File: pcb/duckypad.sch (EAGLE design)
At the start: 159 parts, among them IC2 REG1117, SW1 SPST_TACT-EVQQ2, SW2 SPST_TACT-EVQQ2, SW21 EC12E_SW, SW22 EC12E_SW, SW3 324_SW324_SWITCH_FOOT_HOLE, SW4 324_SW324_SWITCH_FOOT_HOLE, U1 USBC_16P, U2 USBC_16P, U3 ESP32-S3FN8, U5 W25Q32FVSS, X3 SM12B-SSR-H-TB, Y1 16MHz_12pF

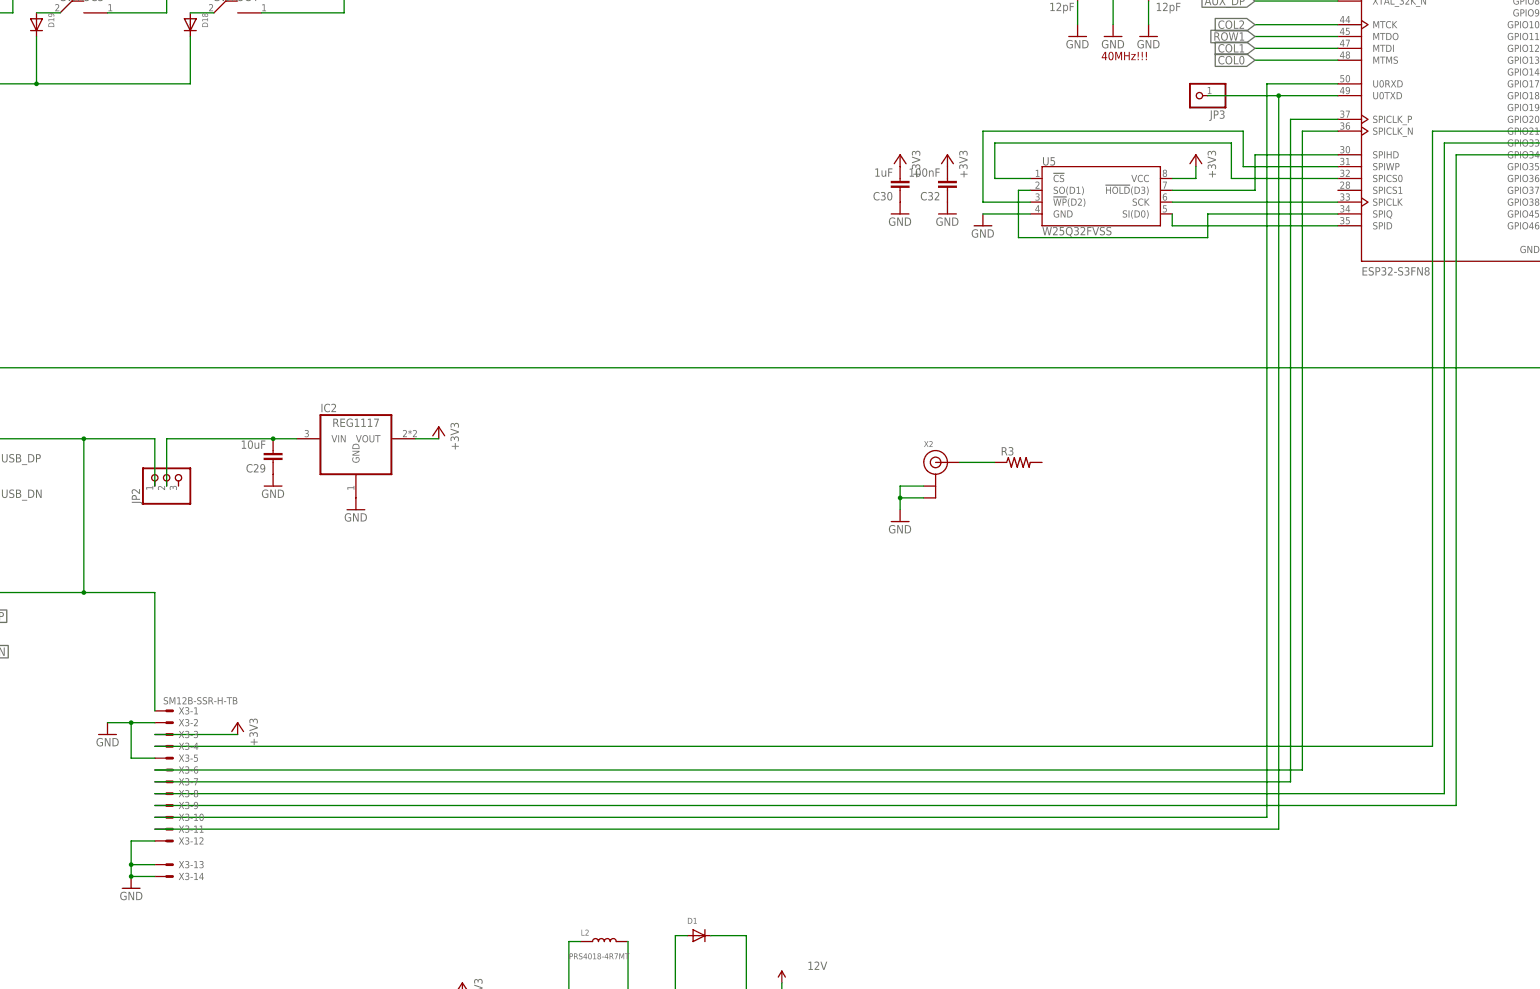
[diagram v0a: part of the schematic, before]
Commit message: finishing touches
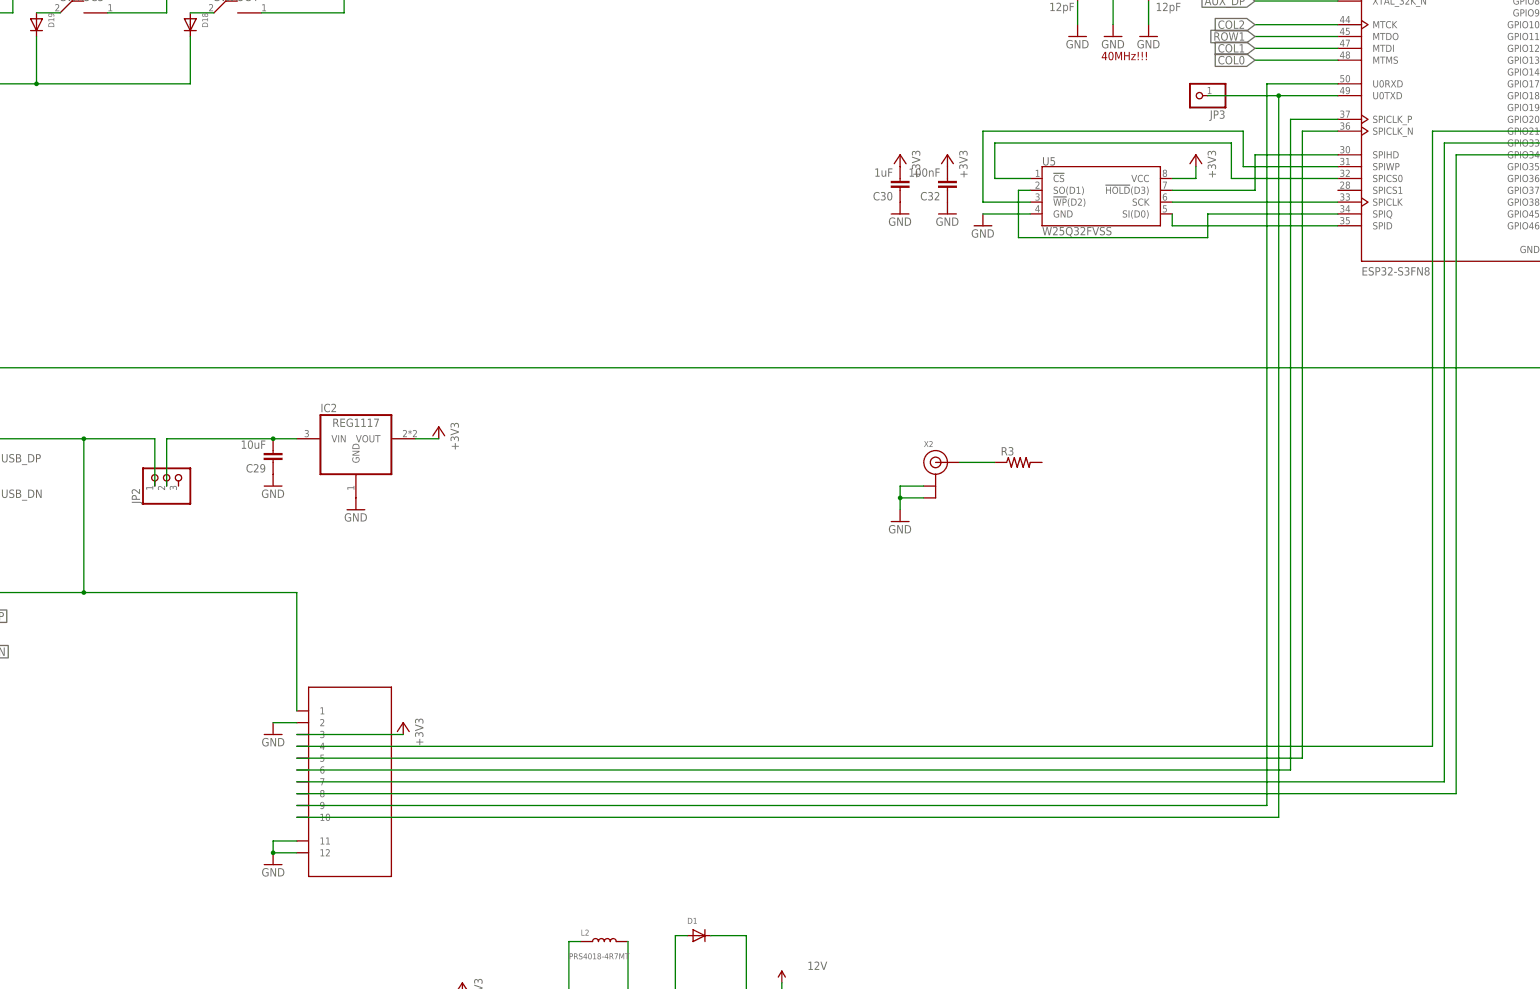
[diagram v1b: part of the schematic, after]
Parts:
- removed X3: SM12B-SSR-H-TB, duckypad:SM12B-SSR-H-TB
- added U$3: SH10P, duckypad:SH10P
- D1, D10, D11, D12, D13, D14, D15, D16, D17, D18, D19, D2, D20, D21, D3, D4, D5, D6, D7, D8, D9: device adafruit_changed:DIODESOD-123 -> duckypad:ADAFRUIT_CHANGED_DIODESOD-123
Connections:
- net +3V3: now also U$3.3; no longer X3-3.S
- net GND: now also U$3.11, U$3.12, U$3.2; no longer X3-12.S, X3-13.S, X3-14.S, X3-2.S, X3-5.S
- net N$1: now also U$3.1; no longer X3-1.S
- net N$37: now also U$3.4; no longer X3-4.S
- net N$67: now also U$3.5; no longer X3-6.S
- net N$68: now also U$3.6; no longer X3-7.S
- net N$69: now also U$3.7; no longer X3-8.S
- net N$70: now also U$3.8; no longer X3-9.S
- net N$72: now also U$3.9; no longer X3-10.S
- net N$73: now also U$3.10; no longer X3-11.S
